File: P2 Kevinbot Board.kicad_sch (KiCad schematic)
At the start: 1 part, among them U1 P2_EDGE_MODULE_SOCKET

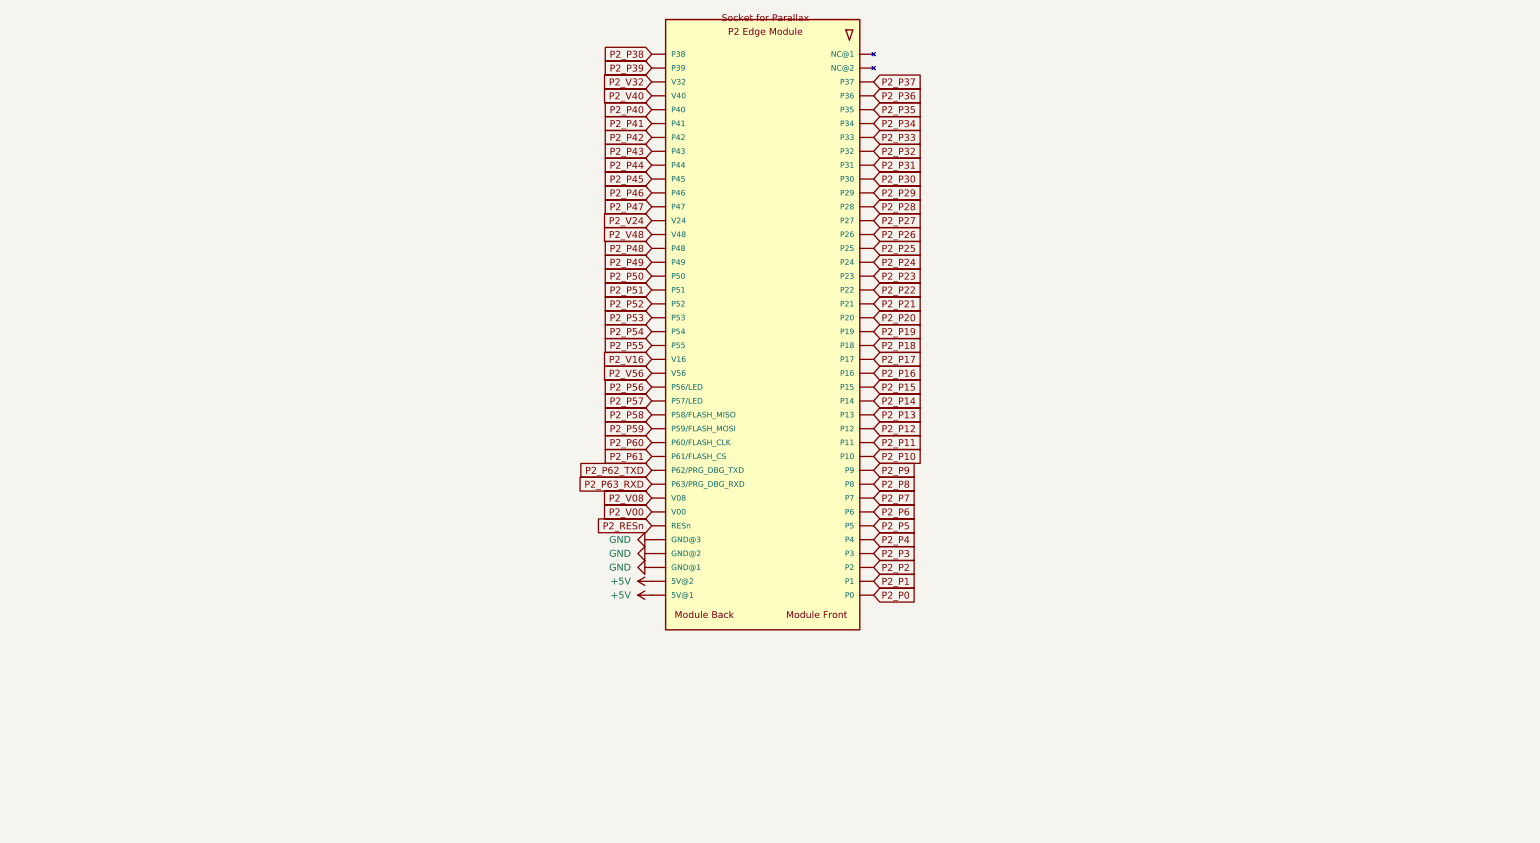
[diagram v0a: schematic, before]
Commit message: Mostly routed accessory headers
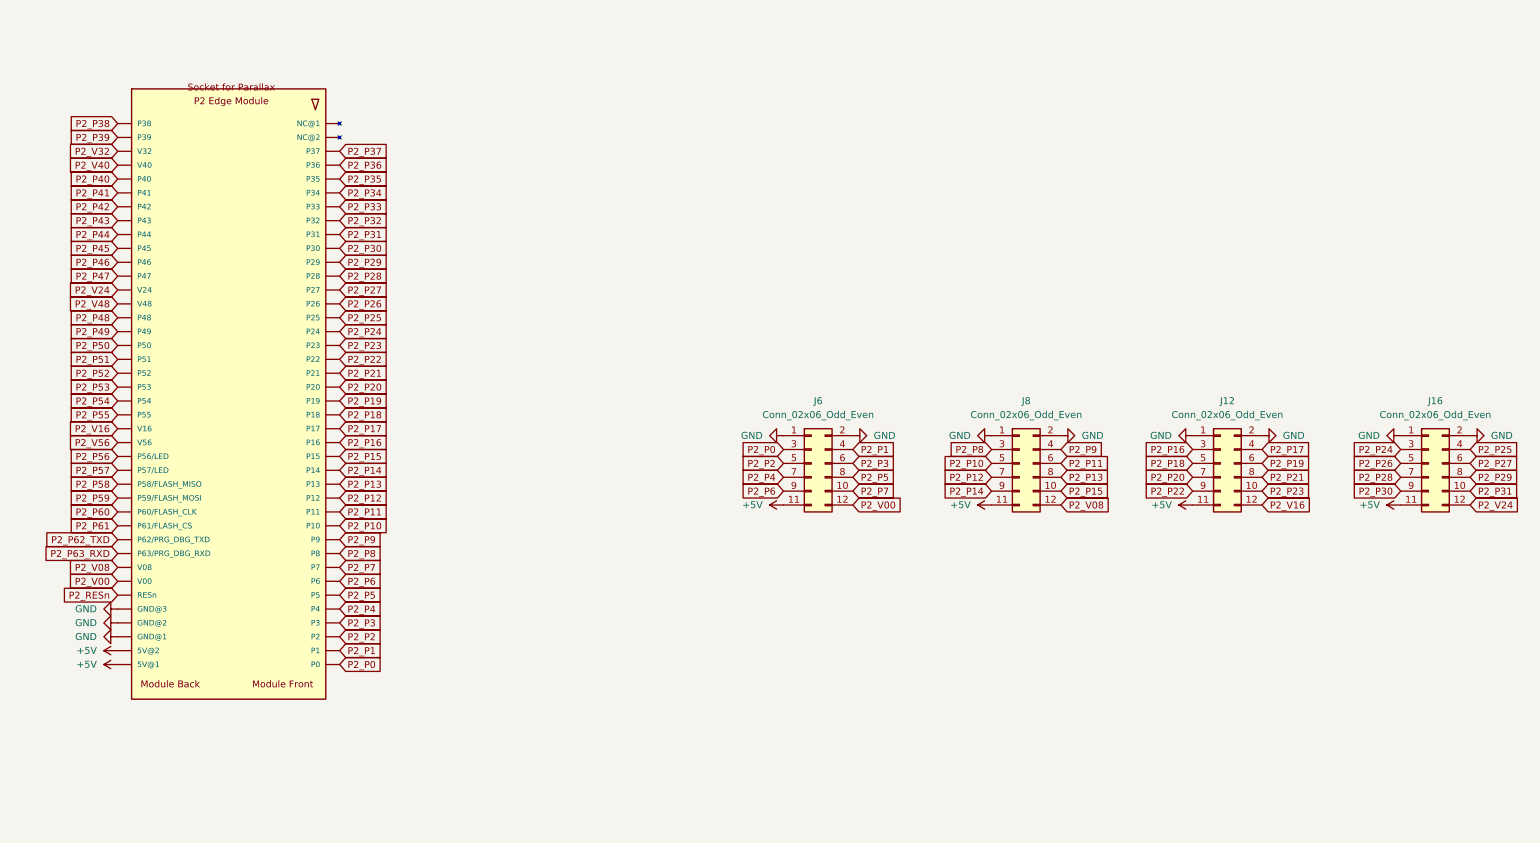
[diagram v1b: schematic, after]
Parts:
- added J12, J16, J6, J8: Conn_02x06_Odd_Even, Connector_PinHeader_2.54mm:PinHeader_2x06_P2.54mm_Vertical, symbol Connector_Generic:Conn_02x06_Odd_Even
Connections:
- net +5V: now also J12.11 (Pin_11), J16.11 (Pin_11), J6.11 (Pin_11), J8.11 (Pin_11)
- net GND: now also J12.1 (Pin_1), J12.2 (Pin_2), J16.1 (Pin_1), J16.2 (Pin_2), J6.1 (Pin_1), J6.2 (Pin_2), J8.1 (Pin_1), J8.2 (Pin_2)
- net P2_P0: now also J6.3 (Pin_3)
- net P2_P1: now also J6.4 (Pin_4)
- net P2_P10: now also J8.5 (Pin_5)
- net P2_P11: now also J8.6 (Pin_6)
- net P2_P12: now also J8.7 (Pin_7)
- net P2_P13: now also J8.8 (Pin_8)
- net P2_P14: now also J8.9 (Pin_9)
- net P2_P15: now also J8.10 (Pin_10)
- net P2_P16: now also J12.3 (Pin_3)
- net P2_P17: now also J12.4 (Pin_4)
- net P2_P18: now also J12.5 (Pin_5)
- net P2_P19: now also J12.6 (Pin_6)
- net P2_P2: now also J6.5 (Pin_5)
- net P2_P20: now also J12.7 (Pin_7)
- net P2_P21: now also J12.8 (Pin_8)
- net P2_P22: now also J12.9 (Pin_9)
- net P2_P23: now also J12.10 (Pin_10)
- net P2_P24: now also J16.3 (Pin_3)
- net P2_P25: now also J16.4 (Pin_4)
- net P2_P26: now also J16.5 (Pin_5)
- net P2_P27: now also J16.6 (Pin_6)
- net P2_P28: now also J16.7 (Pin_7)
- net P2_P29: now also J16.8 (Pin_8)
- net P2_P3: now also J6.6 (Pin_6)
- net P2_P30: now also J16.9 (Pin_9)
- net P2_P31: now also J16.10 (Pin_10)
- net P2_P4: now also J6.7 (Pin_7)
- net P2_P5: now also J6.8 (Pin_8)
- net P2_P6: now also J6.9 (Pin_9)
- net P2_P7: now also J6.10 (Pin_10)
- net P2_P8: now also J8.3 (Pin_3)
- net P2_P9: now also J8.4 (Pin_4)
- net P2_V00: now also J6.12 (Pin_12)
- net P2_V08: now also J8.12 (Pin_12)
- net P2_V16: now also J12.12 (Pin_12)
- net P2_V24: now also J16.12 (Pin_12)

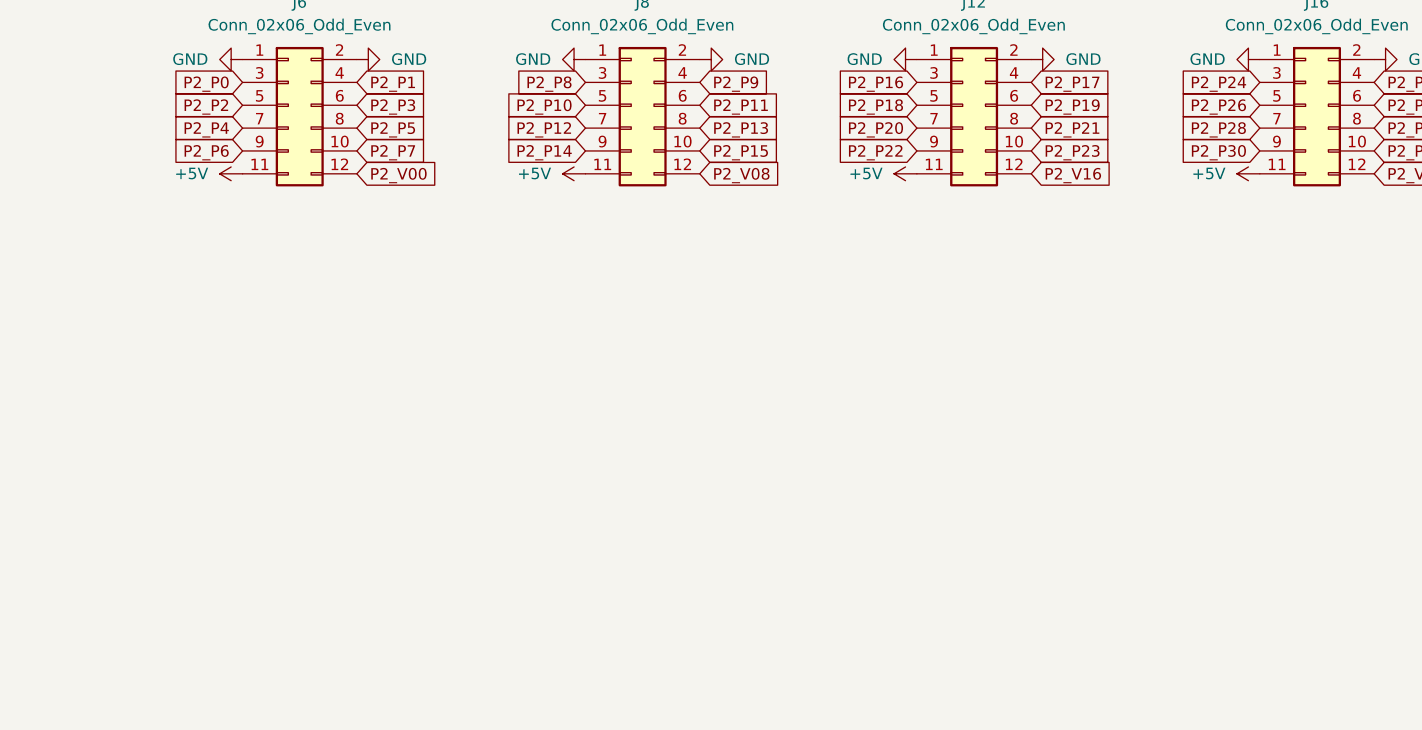
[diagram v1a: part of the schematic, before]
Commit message: Begin work on usbc programmer, misc
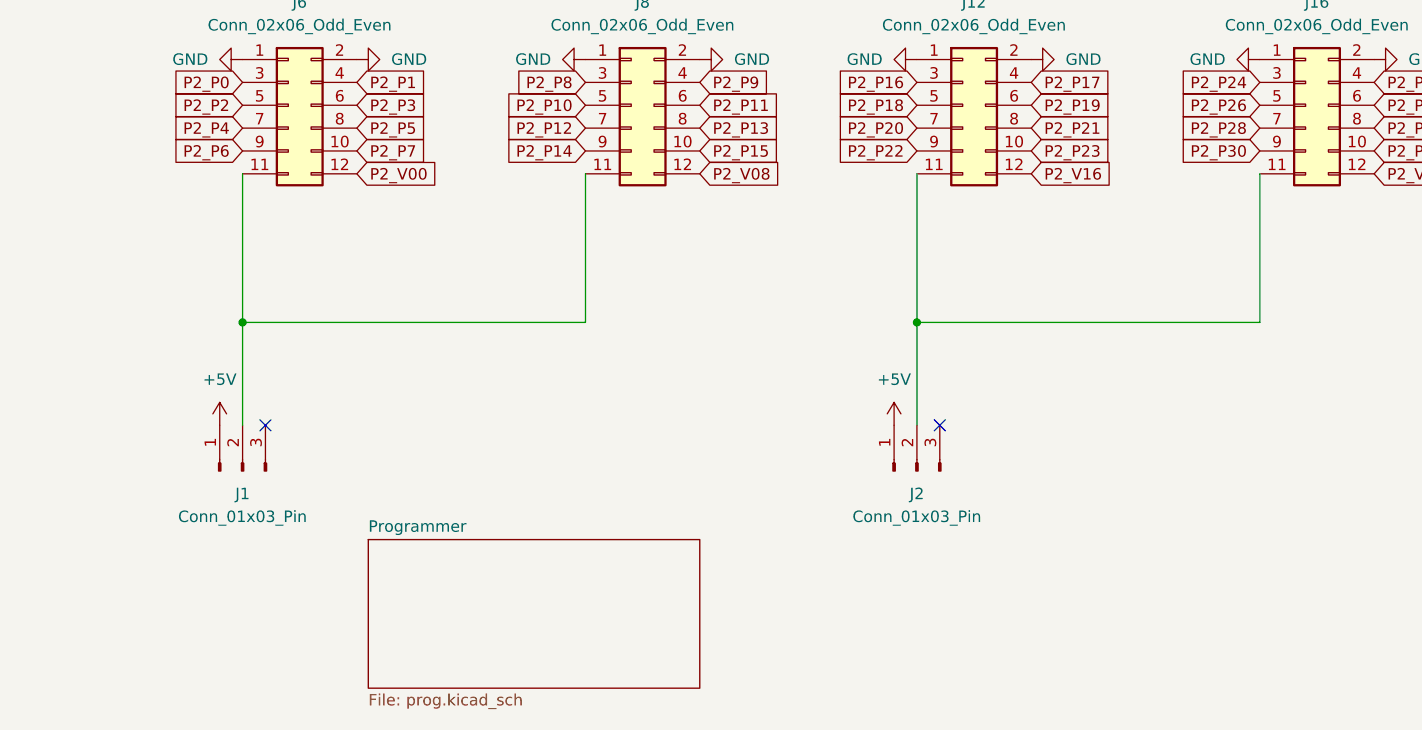
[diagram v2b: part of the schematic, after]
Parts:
- added J1, J2: Conn_01x03_Pin, Connector_PinHeader_2.54mm:PinHeader_1x03_P2.54mm_Vertical, symbol Connector:Conn_01x03_Pin
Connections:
- net +5V: now also J1.1 (Pin_1), J2.1 (Pin_1); no longer J12.11 (Pin_11), J16.11 (Pin_11), J6.11 (Pin_11), J8.11 (Pin_11)
- new net: J12.11 (Pin_11), J16.11 (Pin_11), J2.2 (Pin_2)
- new net: J1.2 (Pin_2), J6.11 (Pin_11), J8.11 (Pin_11)
- no-connect marks 0 -> 2
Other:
- added sheet Programmer (prog.kicad_sch)

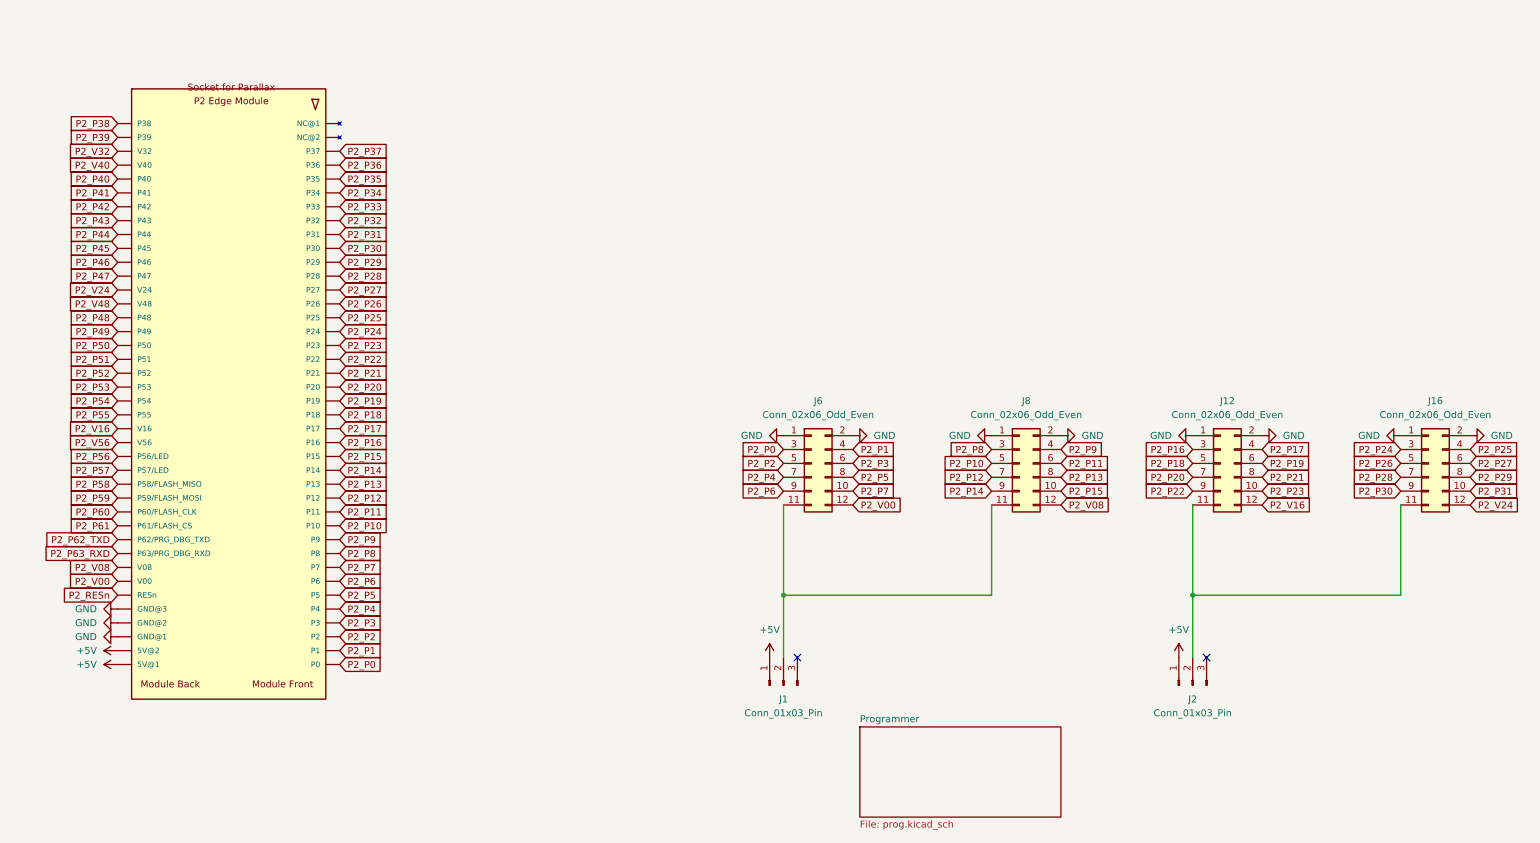
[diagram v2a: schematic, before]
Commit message: Usb programme
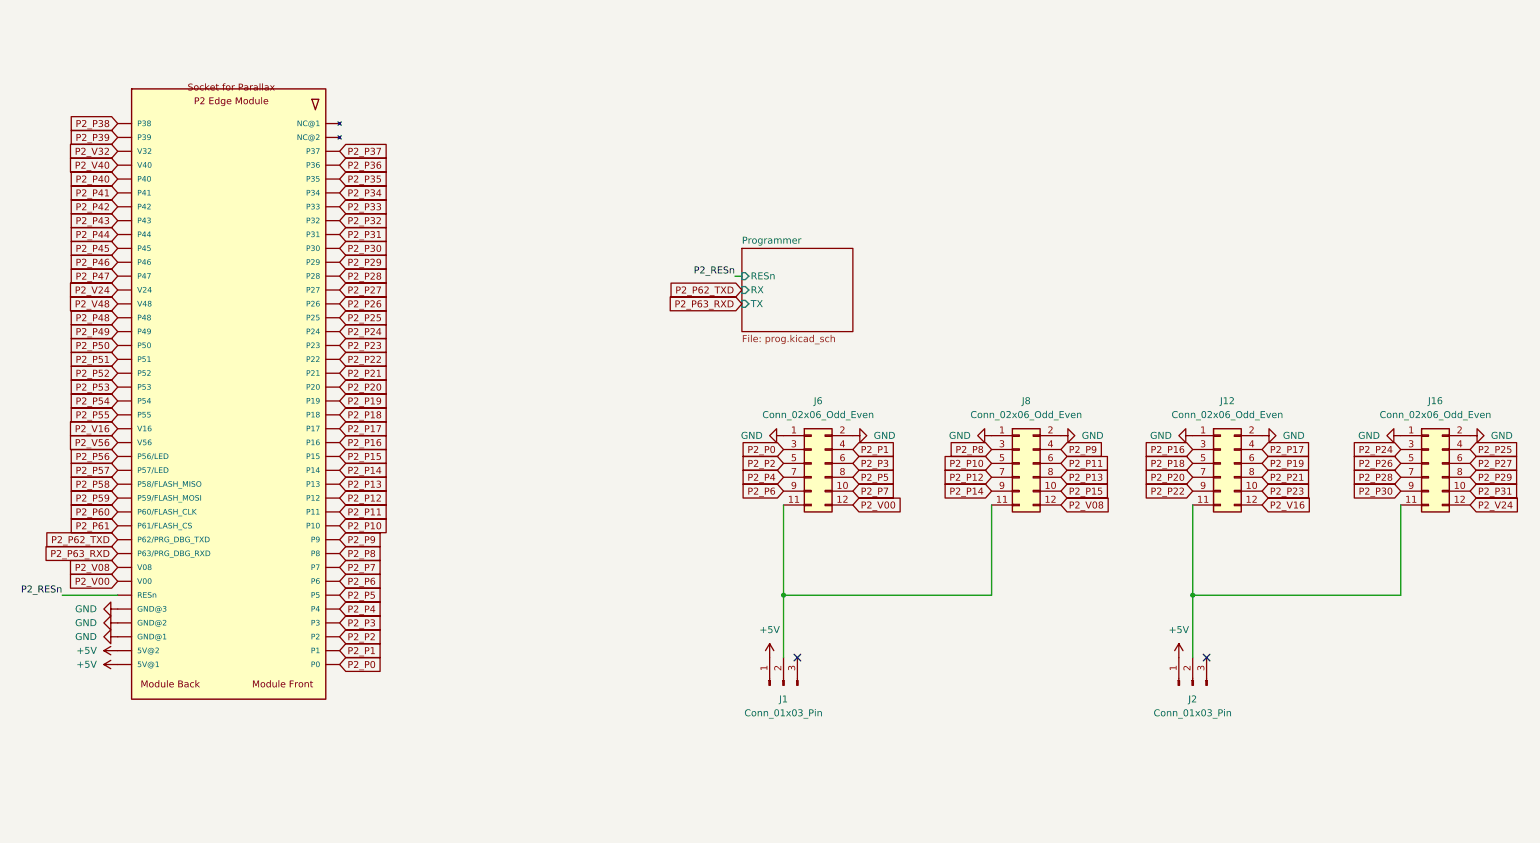
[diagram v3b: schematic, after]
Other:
- sheet Programmer ports: added RESn, RX, TX; removed none
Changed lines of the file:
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@@
 	(wire
 		(pts
+			(xy 39.37 147.32) (xy 49.53 147.32)
+		)
+		(stroke
+			(width 0)
+			(type default)
+		)
+	)
+	(wire
+		(pts
 			(xy 171.45 147.32) (xy 171.45 158.75)
 		)
@@
 	(wire
 		(pts
+			(xy 162.56 88.9) (xy 163.83 88.9)
+		)
+		(stroke
+			(width 0)
+			(type default)
+		)
+	)
+	(wire
+		(pts
 			(xy 284.48 147.32) (xy 284.48 130.81)
 		)
@@
 		)
 	)
+	(label "P2_RESn"
+		(at 162.56 88.9 180)
+		(effects
+			(font
+				(size 1.27 1.27)
+			)
+			(justify right bottom)
+		)
+	)
+	(label "P2_RESn"
+		(at 39.37 147.32 180)
+		(effects
+			(font
+				(size 1.27 1.27)
+			)
+			(justify right bottom)
+		)
+	)
 	(global_label "P2_P31"
 		(shape input)
@@
 		)
 	)
-	(global_label "P2_RESn"
-		(shape input)
-		(at 49.53 147.32 180)
-		(fields_autoplaced yes)
-		(effects
-			(font
-				(size 1.27 1.27)
-			)
-			(justify right)
-		)
-		(property "Intersheetrefs" "${INTERSHEET_REFS}"
-			(at 38.8921 147.2406 0)
-			(effects
-				(font
-					(size 1.27 1.27)
-				)
-				(justify right)
-				(hide yes)
-			)
-		)
-	)
 	(global_label "P2_P16"
 		(shape input)
@@
 		)
 	)
+	(global_label "P2_P62_TXD"
+		(shape input)
+		(at 163.83 91.44 180)
+		(fields_autoplaced yes)
+		(effects
+			(font
+				(size 1.27 1.27)
+			)
+			(justify right)
+		)
+		(property "Intersheetrefs" "${INTERSHEET_REFS}"
+			(at 149.8659 91.5194 0)
+			(effects
+				(font
+					(size 1.27 1.27)
+				)
+				(justify right)
+				(hide yes)
+			)
+		)
+	)
+	(global_label "P2_P63_RXD"
+		(shape input)
+		(at 163.83 93.98 180)
+		(fields_autoplaced yes)
+		(effects
+			(font
+				(size 1.27 1.27)
+			)
+			(justify right)
+		)
+		(property "Intersheetrefs" "${INTERSHEET_REFS}"
+			(at 149.5636 94.0594 0)
+			(effects
+				(font
+					(size 1.27 1.27)
+				)
+				(justify right)
+				(hide yes)
+			)
+		)
+	)
 	(global_label "P2_P7"
 		(shape input)
@@
 	)
 	(sheet
-		(at 185.42 171.45)
-		(size 36.83 16.51)
+		(at 163.83 83.82)
+		(size 20.32 15.24)
 		(exclude_from_sim no)
 		(in_bom yes)
@@
 		)
 		(property "Sheetname" "Programmer"
-			(at 185.42 170.7384 0)
+			(at 163.83 83.1084 0)
 			(effects
 				(font
@@
 		)
 		(property "Sheetfile" "prog.kicad_sch"
-			(at 185.42 188.5446 0)
+			(at 163.83 99.6446 0)
 			(effects
 				(font
@@
 			)
 		)
+		(pin "RESn" input
+			(at 163.83 88.9 180)
+			(effects
+				(font
+					(size 1.27 1.27)
+				)
+				(justify left)
+			)
+		)
+		(pin "RX" input
+			(at 163.83 91.44 180)
+			(effects
+				(font
+					(size 1.27 1.27)
+				)
+				(justify left)
+			)
+		)
+		(pin "TX" input
+			(at 163.83 93.98 180)
+			(effects
+				(font
+					(size 1.27 1.27)
+				)
+				(justify left)
+			)
+		)
